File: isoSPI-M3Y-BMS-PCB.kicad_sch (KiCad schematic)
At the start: 427 parts, among them J1 Screw_Terminal_01x04, J10 Screw_Terminal_01x04, J11 Screw_Terminal_01x03, J12 Screw_Terminal_01x08, J13 Conn_02x10_Odd_Even, J14 Screw_Terminal_01x04, J15 USB_C_Receptacle_USB2.0_16P, J16 Conn_01x03, J17 USB_C_Receptacle_USB2.0_16P, J18 USB_C_Receptacle_USB2.0_16P, J2 Conn_02x10_Odd_Even, J3 8P8C_LED_Shielded_x2, J5 OEM Shunt Connector, J6 349128020, J7 OEM HV Sense Connector, J8 OEM Connector, J9 Conn_01x03, K10 FC Positive, K11 FC Negative, K12 Link Negative, K13 Inverter, K14 Link Positive, K15 Link Negative, K16 FC Positive, K17 FC Negative, K18 Inverter, K9 Link Positive, Q1 CRSM034N06L2, Q2 CRSM034N06L2, Q3 CRSM034N06L2, Q5 CRSM034N06L2, SW1 TS-1187A-B-A-B, SW2 TS-1187A-B-A-B, SW3 TS-1187A-B-A-B, SW4 TS-1187A-B-A-B, U1 SN74LV1T08DBVR, U10 LTV-217-B-G, U11 RP2354B, U12 ADS1115, U13 ISO1050DUB, U15 SN74LV1T08DBVR, U16 BatMan, U17 TPS5430DDAR, U2 ISO1540, U20 LTV-217-B-G, U21 AMS1117-3.3, U22 F0505S-1WR3, U23 SN74LV1T08DBVR, U24 F0505S-1WR3, U25 SN74LV1T08DBVR, U26 SN74LV1T08DBVR, U27 RP2354B, U28 AM26LV32EIDR, U29 B0505S-3WR2, U3 INA228, U30 ISO1540, U32 SP3485EN-L/TR, U4 ISO1540, U6 F0505S-1WR3, U8 LTV-217-B-G, U9 LTV-217-B-G, Y1 ABM8-272-T3, Y2 ABM8-272-T3

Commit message: getting close!
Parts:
- removed C27: 4.7u, Capacitor_SMD:C_0402_1005Metric, symbol Device:C
- removed R50: 33r, Resistor_SMD:R_0402_1005Metric, symbol Device:R
- added C27, C90: 1uF, Capacitor_SMD:C_0603_1608Metric, symbol Device:C_Small
- added C77, C83, C84, C88: 100nF, Capacitor_SMD:C_0603_1608Metric, symbol Device:C_Small
- added D35: White, LED_SMD:LED_0805_2012Metric, symbol Device:LED
- added R50, R73: 10k, Resistor_SMD:R_0603_1608Metric_Pad0.98x0.95mm_HandSolder, symbol Device:R_Small
- added R71, R72: 1.8k, Resistor_SMD:R_0603_1608Metric, symbol Device:R_Small
- added R76: 24k, Resistor_SMD:R_0603_1608Metric, symbol Device:R_Small
- added TP20, TP21: TestPoint_2Pole, BMS_Library:TestPoint_2Pads_Pitch2.54mm_Pad1.5_Drill1.0mm, symbol Connector:TestPoint_2Pole
- added U5, U7: LTV-217-B-G, Package_SO:SSOP-4_4.4x2.6mm_P1.27mm, symbol Isolator:LTV-817S
- C26, C40: footprint Capacitor_SMD:C_0603_1608Metric_Pad1.08x0.95mm_HandSolder -> Capacitor_SMD:C_0603_1608Metric
- U22, U24, U6: footprint Converter_DCDC:Converter_DCDC_TRACO_TEA1-xxxxHI_THT -> BMS_Library:H0505S-1WR2
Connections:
- net +3.3V: now also R80.2, U5.4, U7.4
- net +5V: now also C27.2, C90.2, U5.1, U7.1
- net 3.3V Sense: now also C83.2
- net 5V Sense: now also C84.2
- net GND: now also J8.3 (Pin_3), J8.4 (Pin_4), C77.1, C83.1, C84.1, C88.1, D35.1 (K), R50.1, R73.1, TP20.1, TP21.1
- net HMI Serial RX: now also R34.1, U27.47 (GPIO38); no longer R35.1, U27.48 (GPIO39)
- net HMI Serial TX: now also R35.1, U27.48 (GPIO39); no longer R34.1, U27.47 (GPIO38)
- net IsoSPI RX Debug: no longer U11.39 (GPIO31)
- net Snooper Debug: no longer U11.40 (GPIO32)
- net VContactor Sense: now also C77.2
- net V_{Contactor}: now also R76.1
- net Vin Logic Sense: now also C88.2
- net 1/2 Vsense: now reaches C10.1, C41.2, C42.1, C43.2, C95.2, R228.2, R229.1, R40.2, R41.1, R45.2, R47.1
- net at J8.17 (Pin_17): now also R72.1
- net at J8.18 (Pin_18): now also R71.1
- net GPIO10 renamed FC-CTR-POS-AUX
- net FC-CTR-POS-AUX: now also R50.2, U5.3
- net GPIO9 renamed FC-CTR-NEG-AUX
- net FC-CTR-NEG-AUX: now also R73.2, U7.3
- new net: D35.2 (A), R76.2
- new net: C90.1, R72.2, U7.2
- new net: C27.1, R71.2, U5.2
- new net IsoSPI RX Debug 2: TP20.2, U11.39 (GPIO31)
- new net Snooper Debug 2: TP21.2, U11.40 (GPIO32)
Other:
- note added: "Specified DC-DC is a smaller package - put footprint will fit the 3KV or 6KV version"
- moved on the sheet: C26, C40, D18, D50, D51, J12, J3B, J8, R22, R23, R28, R29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

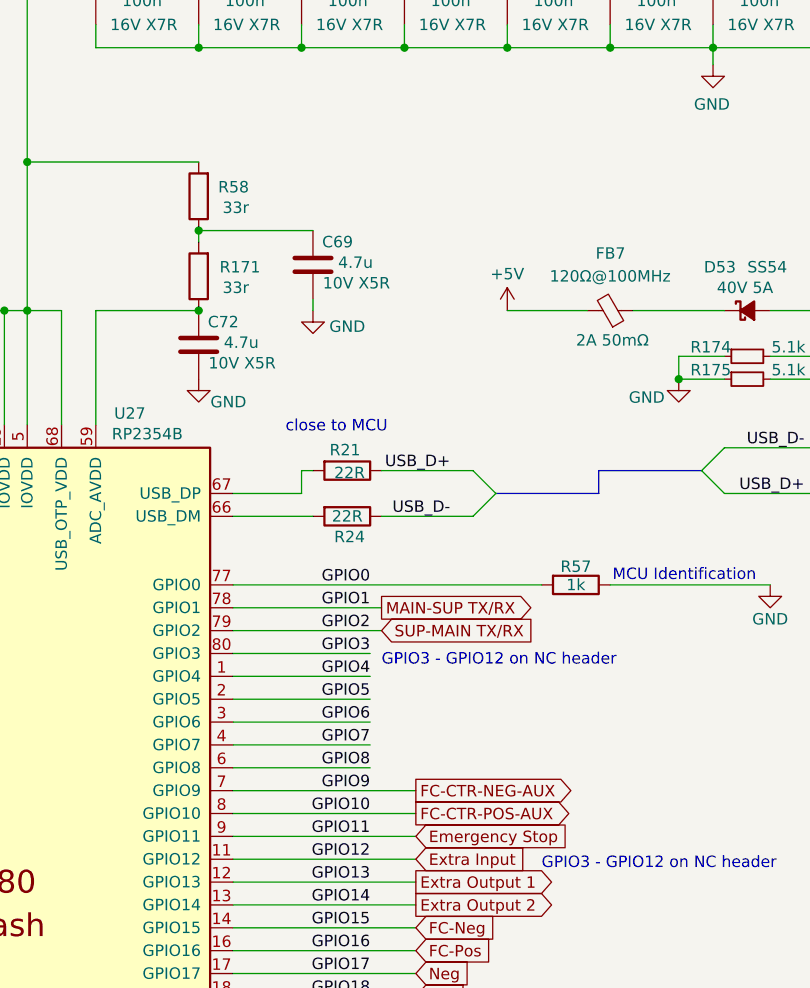
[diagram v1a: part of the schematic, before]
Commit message: progress
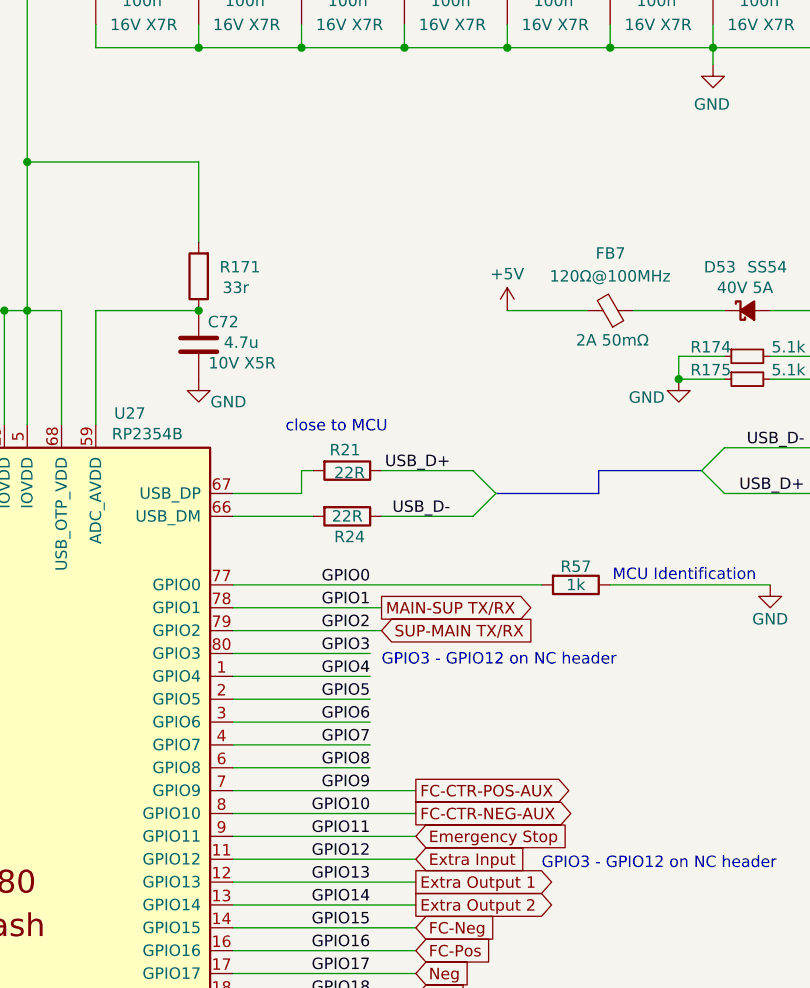
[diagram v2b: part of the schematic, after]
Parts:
- removed C69: 4.7u, Capacitor_SMD:C_0402_1005Metric, symbol Device:C
- removed R58: 33r, Resistor_SMD:R_0402_1005Metric, symbol Device:R
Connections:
- net +3.3V: now also R171.2
- net FC-CTR-NEG-AUX: now also J2.16 (Pin_16), U27.8 (GPIO10); no longer J2.14 (Pin_14), U27.7 (GPIO9)
- net FC-CTR-POS-AUX: now also J2.14 (Pin_14), U27.7 (GPIO9); no longer J2.16 (Pin_16), U27.8 (GPIO10)
